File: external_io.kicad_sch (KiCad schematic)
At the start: 19 parts, among them J1 UJ20-C-H-G-SMT-1-P16-TR, J2 Conn_01x02_Socket, J3 Conn_01x03_Socket, J4 Conn_01x04_Socket, J5 Conn_01x03_Socket, J6 Conn_01x03_Socket, U1 USBLC6-2SC6, U2 USBLC6-2SC6

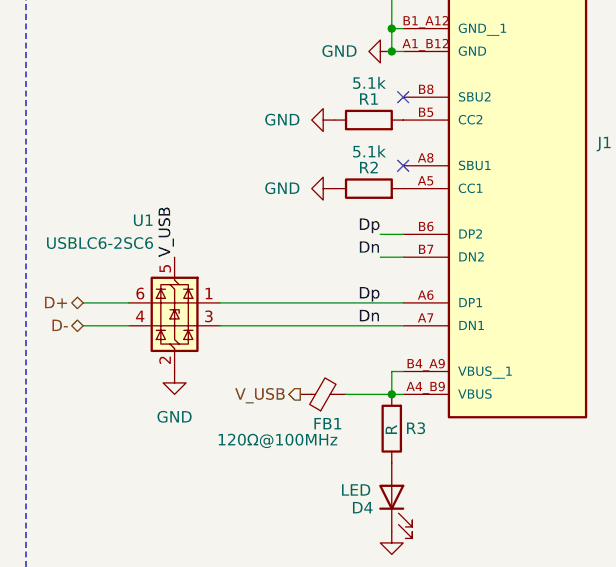
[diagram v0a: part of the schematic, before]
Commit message: Redoing layout
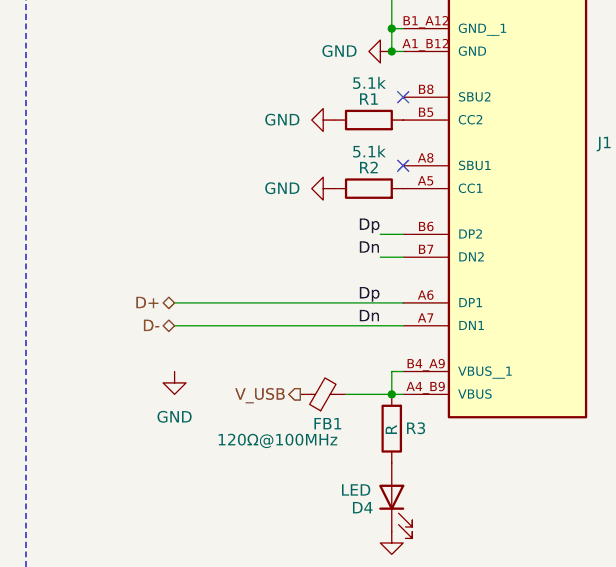
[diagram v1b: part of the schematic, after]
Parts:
- removed U1: USBLC6-2SC6, Package_TO_SOT_SMD:SOT-23-6, symbol Power_Protection:USBLC6-2SC6
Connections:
- net Dn is gone; now on net D-: J1.A7 (DN1), J1.B7 (DN2)
- net Dp is gone; now on net D+: J1.A6 (DP1), J1.B6 (DP2)
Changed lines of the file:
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@@
 	(wire
 		(pts
-			(xy 22.86 74.93) (xy 27.94 74.93)
+			(xy 33.02 74.93) (xy 58.42 74.93)
 		)
 		(stroke
@@
 		)
 	)
-	(wire
-		(pts
-			(xy 38.1 74.93) (xy 58.42 74.93)
-		)
-		(stroke
-			(width 0)
-			(type default)
-		)
-	)
 	(bus
 		(pts
@@
 	(wire
 		(pts
-			(xy 38.1 77.47) (xy 58.42 77.47)
-		)
-		(stroke
-			(width 0)
-			(type default)
-		)
-	)
-	(wire
-		(pts
 			(xy 57.15 82.55) (xy 58.42 82.55)
 		)
@@
 	(wire
 		(pts
-			(xy 22.86 77.47) (xy 27.94 77.47)
+			(xy 33.02 77.47) (xy 58.42 77.47)
 		)
 		(stroke
@@
 		)
 	)
-	(label "V_USB"
-		(at 33.02 69.85 90)
-		(effects
-			(font
-				(size 1.27 1.27)
-			)
-			(justify left bottom)
-		)
-	)
 	(label "SWDIO"
 		(at 214.63 92.71 0)
@@
 	(hierarchical_label "D+"
 		(shape bidirectional)
-		(at 22.86 74.93 180)
+		(at 33.02 74.93 180)
 		(effects
 			(font
@@
 	(hierarchical_label "D-"
 		(shape bidirectional)
-		(at 22.86 77.47 180)
+		(at 33.02 77.47 180)
 		(effects
 			(font
@@
 					(unit 1)
 				)
-			)
-		)
-	)
-	(symbol
-		(lib_id "Power_Protection:USBLC6-2SC6")
-		(at 33.02 74.93 0)
-		(mirror y)
-		(unit 1)
-		(exclude_from_sim no)
-		(in_bom yes)
-		(on_board yes)
-		(dnp no)
-		(property "Reference" "U1"
-			(at 30.734 65.786 0)
-			(effects
-				(font
-					(size 1.27 1.27)
-				)
-				(justify left)
-			)
-		)
-		(property "Value" "USBLC6-2SC6"
-			(at 30.734 68.326 0)
-			(effects
-				(font
-					(size 1.27 1.27)
-				)
-				(justify left)
-			)
-		)
-		(property "Footprint" "Package_TO_SOT_SMD:SOT-23-6"
-			(at 31.75 81.28 0)
-			(effects
-				(font
-					(size 1.27 1.27)
-					(italic yes)
-				)
-				(justify left)
-				(hide yes)
-			)
-		)
-		(property "Datasheet" "https://www.st.com/resource/en/datasheet/usblc6-2.pdf"
-			(at 31.75 83.185 0)
-			(effects
-				(font
-					(size 1.27 1.27)
-				)
-				(justify left)
-				(hide yes)
-			)
-		)
-		(property "Description" "Very low capacitance ESD protection diode, 2 data-line, SOT-23-6"
-			(at 33.02 74.93 0)
-			(effects
-				(font
-					(size 1.27 1.27)
-				)
-				(hide yes)
-			)
-		)
-		(property "Mfr" "STMicroelectronics"
-			(at 33.02 74.93 0)
-			(effects
-				(font
-					(size 1.27 1.27)
-				)
-				(hide yes)
-			)
-		)
-		(property "Mfr P/N" "USBLC6-2SC6"
-			(at 33.02 74.93 0)
-			(effects
-				(font
-					(size 1.27 1.27)
-				)
-				(hide yes)
-			)
-		)
-		(property "Supplier_1" "Digikey"
-			(at 33.02 74.93 0)
-			(effects
-				(font
-					(size 1.27 1.27)
-				)
-				(hide yes)
-			)
-		)
-		(property "Supplier_1 P/N" "497-5235-2-ND"
-			(at 33.02 74.93 0)
-			(effects
-				(font
-					(size 1.27 1.27)
-				)
-				(hide yes)
-			)
-		)
-		(property "Supplier_1 Unit Price" "0.36000"
-			(at 33.02 74.93 0)
-			(effects
-				(font
-					(size 1.27 1.27)
-				)
-				(hide yes)
-			)
-		)
-		(property "Supplier_1 Price @ Qty" "1"
-			(at 33.02 74.93 0)
-			(effects
-				(font
-					(size 1.27 1.27)
-				)
-				(hide yes)
-			)
-		)
-		(property "Supplier_2" "JLCPCB"
-			(at 33.02 74.93 0)
-			(effects
-				(font
-					(size 1.27 1.27)
-				)
-				(hide yes)
-			)
-		)
-		(property "Supplier_2 P/N" "C7519"
-			(at 33.02 74.93 0)
-			(effects
-				(font
-					(size 1.27 1.27)
-				)
-				(hide yes)
-			)
-		)
-		(property "Supplier_2 Unit Price" "0.1373"
-			(at 33.02 74.93 0)
-			(effects
-				(font
-					(size 1.27 1.27)
-				)
-				(hide yes)
-			)
-		)
-		(property "Supplier_2 Price @ Qty" "1"
-			(at 33.02 74.93 0)
-			(effects
-				(font
-					(size 1.27 1.27)
-				)
-				(hide yes)
-			)
-		)
-		(pin "3"
-		)
-		(pin "5"
-		)
-		(pin "1"
-		)
-		(pin "4"
-		)
-		(pin "6"
-		)
-		(pin "2"
-		)
-		(instances
-			(project "BMS"
-				(path "/124184ba-5d68-4d9f-8da6-acc6720ab30b/93f9b420-7cce-46a9-9201-666f07a18f85/2982e12c-39cd-4158-a648-a90b7f6b527c"
-					(reference "U1")
-					(unit 1)
-				)

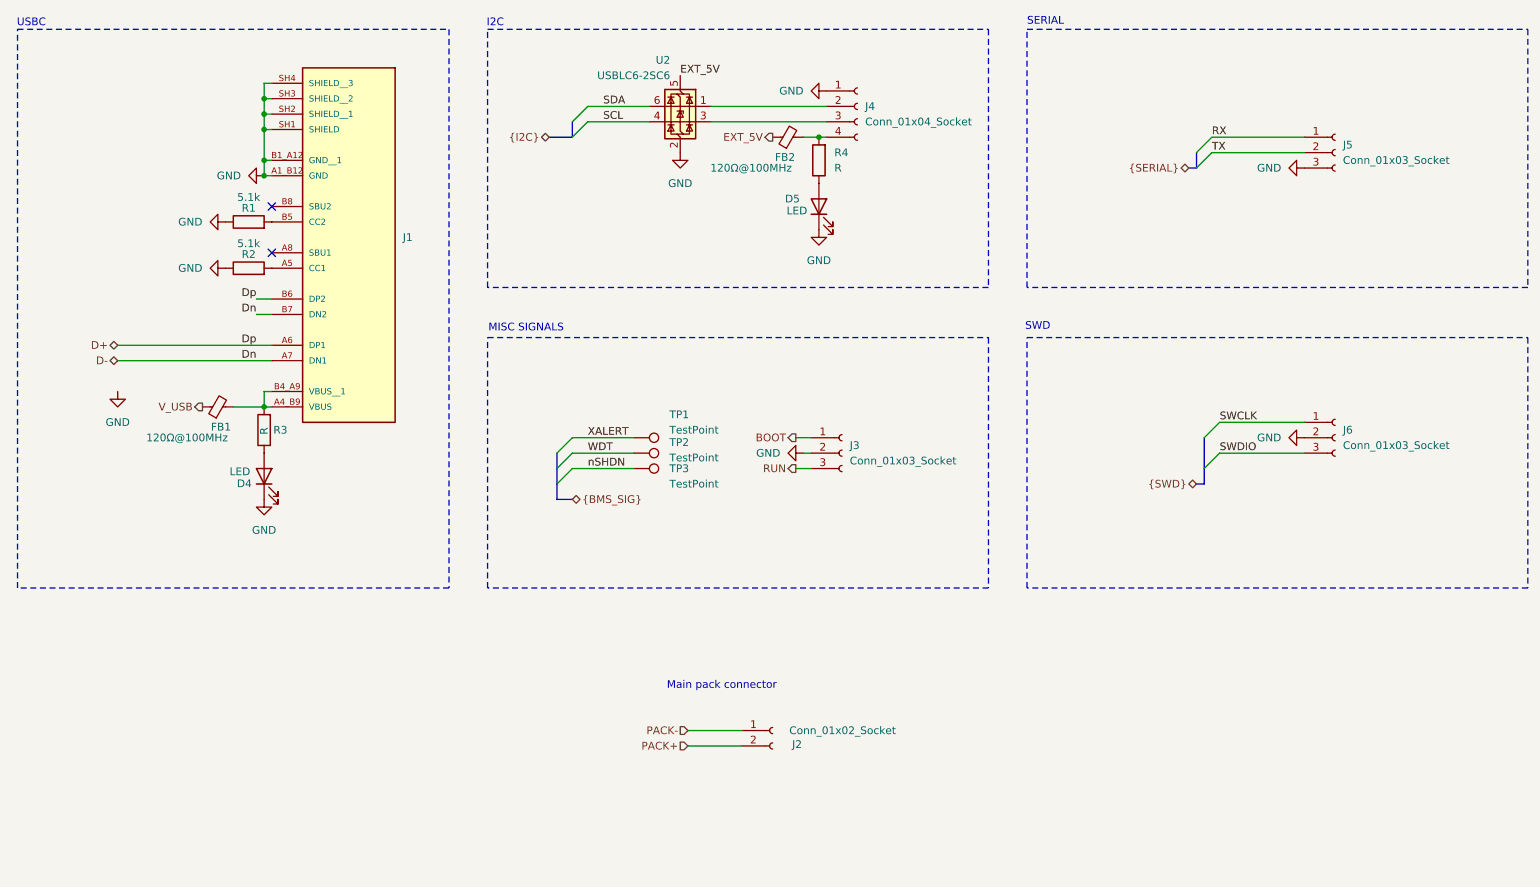
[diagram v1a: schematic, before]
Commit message: prepaing for production
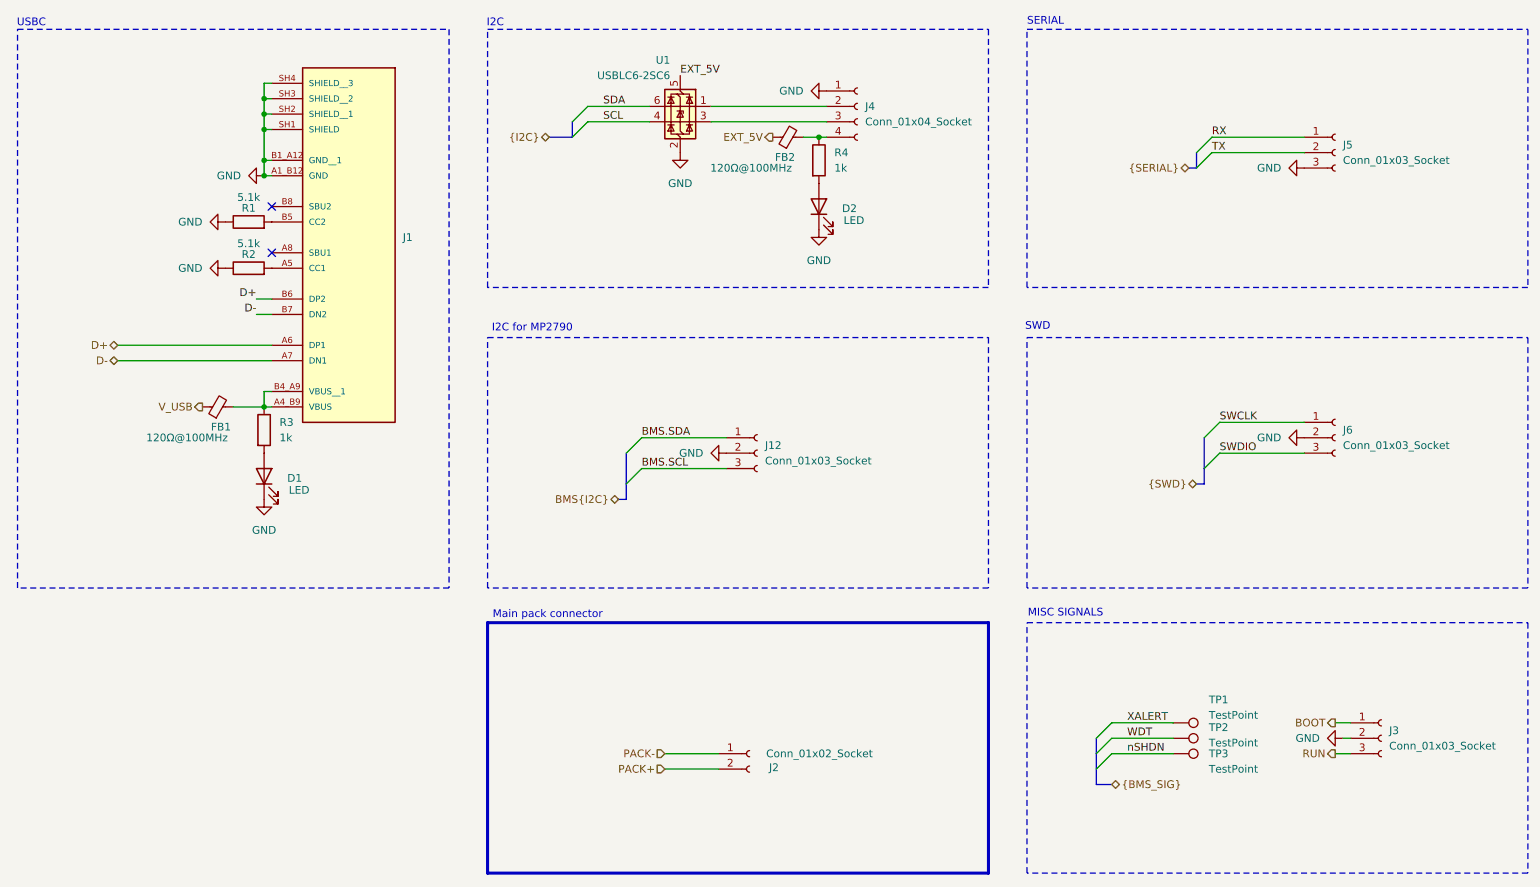
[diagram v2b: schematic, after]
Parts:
- removed D4, D5: LED, symbol Device:LED
- added D1, D2: LED, LED_SMD:LED_0603_1608Metric, symbol Device:LED
- added J12: Conn_01x03_Socket, Connector_PinHeader_2.54mm:PinHeader_1x03_P2.54mm_Vertical, symbol Connector:Conn_01x03_Socket
- J1: Supplier_2 (none) -> JLCPCB; Supplier_2 P/N (none) -> C45082766
- J2: Mfr (none) -> Changzhou Amass Elec; Mfr P/N (none) -> XT30PW-F20.G.Y; Supplier_2 (none) -> JLCPCB; Supplier_2 P/N (none) -> C2913282
- J3, J5, J6: Mfr (none) -> BOOMELE(Boom Precision Elec); Mfr P/N (none) -> 2.54-1*3PPin; Supplier_2 P/N C5116529 -> C49257; Supplier_2 Unit Price 0.0773 -> 0.0209
- J4: Supplier_2 (none) -> JLCPCB
- R3, R4: value R -> 1k; footprint (none) -> Resistor_SMD:R_0603_1608Metric; Mfr (none) -> YAGEO; Mfr P/N (none) -> AC0603FR-071KL; Supplier_2 (none) -> JLCPCB; Supplier_2 P/N (none) -> C116692
- TP1, TP2, TP3: Mfr (none) -> Harwin; Mfr P/N (none) -> S2761-46R; Supplier_2 (none) -> JLCPCB; Supplier_2 P/N (none) -> C5846954
- renumbered U2 to U1
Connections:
- net GND: now also D1.1 (K), D2.1 (K), J12.2 (Pin_2)
- net at FB2.2, J4.4 (Pin_4): now also R4.1; no longer R4.2
- net at FB1.2, J1.A4_B9 (VBUS), J1.B4_A9 (VBUS__1): now also R3.1; no longer R3.2
- new net: D2.2 (A), R4.2
- new net: D1.2 (A), R3.2
- new net BMS.SCL: J12.3 (Pin_3)
- new net BMS.SDA: J12.1 (Pin_1)
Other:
- note added: "I2C for MP2790"
- moved on the sheet: J2, J3, TP1, TP2, TP3
